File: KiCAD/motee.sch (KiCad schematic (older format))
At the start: 49 parts, among them IC1 ATTINY841-MU, J1 SN65HVD3082EDGK, J2 drv8850, U1 TLE4946-2K, U10 pad, U11 pad, U12 pad, U13 pad, U14 pad, U15 pad, U16 pad, U17 MISO, U18 SCK, U19 RESET, U2 TLE4946-2K, U20 pad, U21 MOSI, U22 pad, U23 pad, U24 pad, U25 pad, U26 pad, U27 pad, U28 pad, U29 pad, U3 pad_round, U30 pad, U31 pad, U32 pad, U4 pad_round, U5 pad, U6 pad, U7 pad, U8 pad, U9 pad

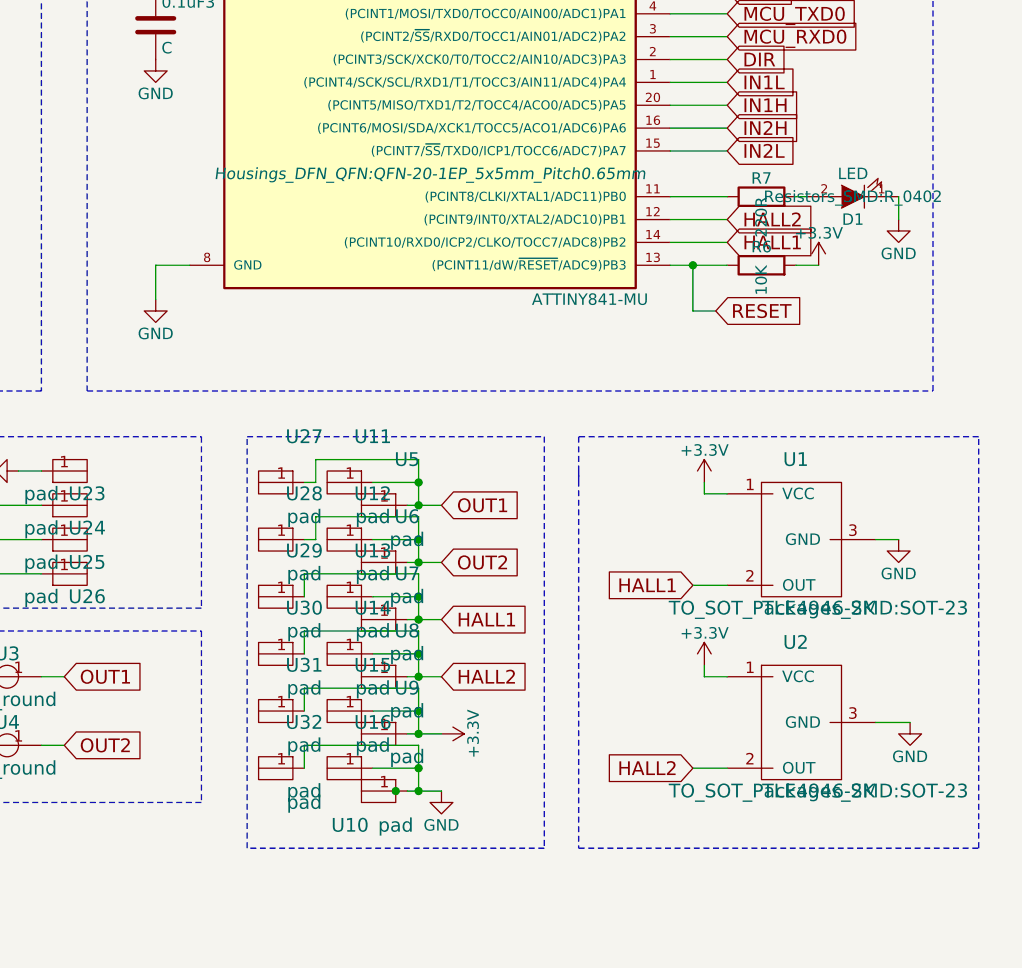
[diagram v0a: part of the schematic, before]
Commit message: poprawki
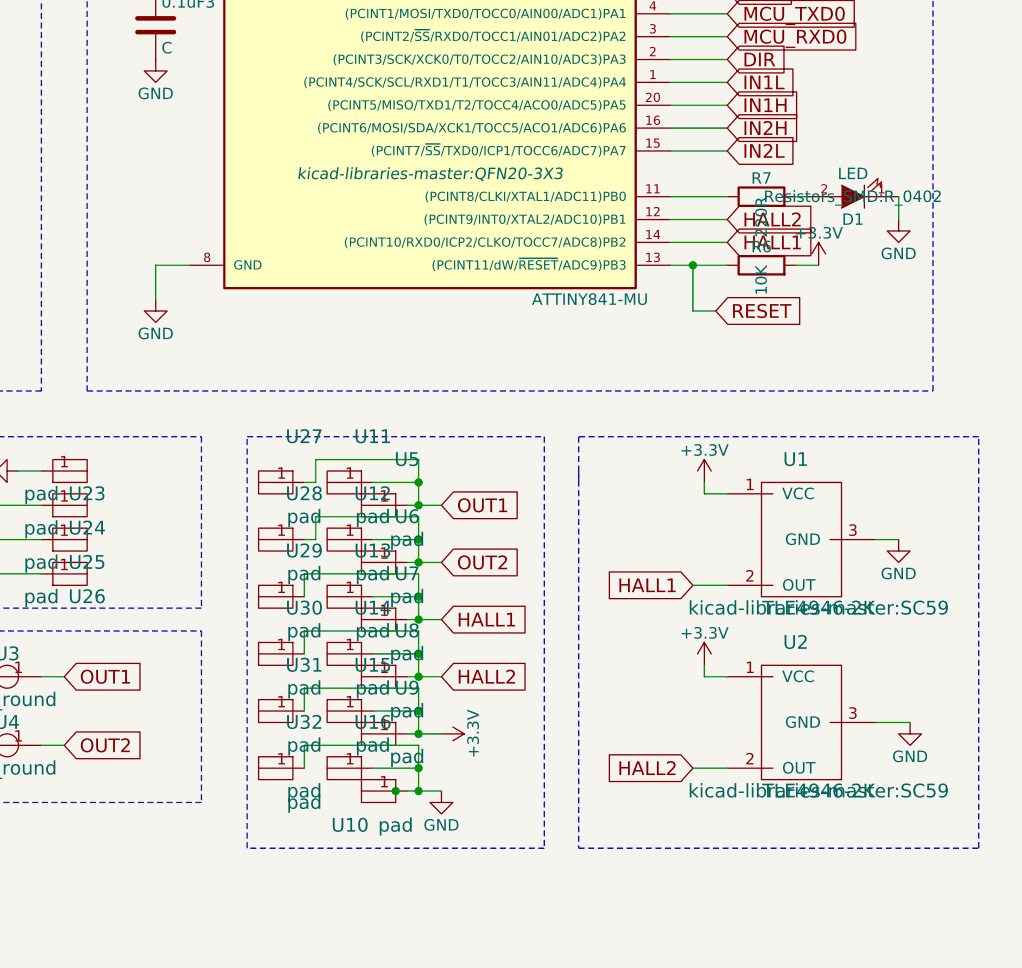
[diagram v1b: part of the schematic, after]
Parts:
- IC1: footprint Housings_DFN_QFN:QFN-20-1EP_5x5mm_Pitch0.65mm -> kicad-libraries-master:QFN20-3X3
- U1, U2: footprint TO_SOT_Packages_SMD:SOT-23 -> kicad-libraries-master:SC59
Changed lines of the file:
@@
 LIBS:TLE4946-2K
 LIBS:pad
-LIBS:motee-cache
 EELAYER 25 0
 EELAYER END
@@
 F 0 "IC1" H 5850 3200 50  0000 C CNN
 F 1 "ATTINY841-MU" H 7400 1700 50  0000 C CNN
-F 2 "Housings_DFN_QFN:QFN-20-1EP_5x5mm_Pitch0.65mm" H 6700 2250 50  0000 C CIN
+F 2 "kicad-libraries-master:QFN20-3X3" H 6700 2250 50  0000 C CIN
 F 3 "" H 6700 2450 50  0000 C CNN
 	1    6700 2450
@@
 F 0 "U1" H 8300 4500 60  0000 C CNN
 F 1 "TLE4946-2K" H 8400 3850 60  0000 C CNN
-F 2 "TO_SOT_Packages_SMD:SOT-23" H 8400 3850 60  0000 C CNN
+F 2 "kicad-libraries-master:SC59" H 8400 3850 60  0000 C CNN
 F 3 "" H 8400 3850 60  0000 C CNN
 	1    8300 4200
@@
 F 0 "U2" H 8300 5300 60  0000 C CNN
 F 1 "TLE4946-2K" H 8400 4650 60  0000 C CNN
-F 2 "TO_SOT_Packages_SMD:SOT-23" H 8400 4650 60  0000 C CNN
+F 2 "kicad-libraries-master:SC59" H 8400 4650 60  0000 C CNN
 F 3 "" H 8400 4650 60  0000 C CNN
 	1    8300 5000
